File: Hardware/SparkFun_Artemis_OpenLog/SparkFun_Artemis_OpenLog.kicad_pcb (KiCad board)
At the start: 4 copper layers, 30.5 x 30.5 mm, 88 parts, among them J11 Qwiic_RA, J14 SWD, J2 Conn_01x02, J3 Conn_01x02, J4 Conn_01x06, J5 JST_2mm_LiPo, J6 MICRO-SD, J7 Conn_01x01, J8 USB_C_Receptacle, Q2 DMG2305UX, SW3 SMD_4.6x2.8mm_h2.5mm, U1 3.0V Supervisor, U10 CH340E, U2 MCP73831, U3 AP2112K-3.3, U4 AP2112K-3.3, U5 BNO086, U8 Artemis Module, Y1 32.768kHz, Y3 32.768kHz

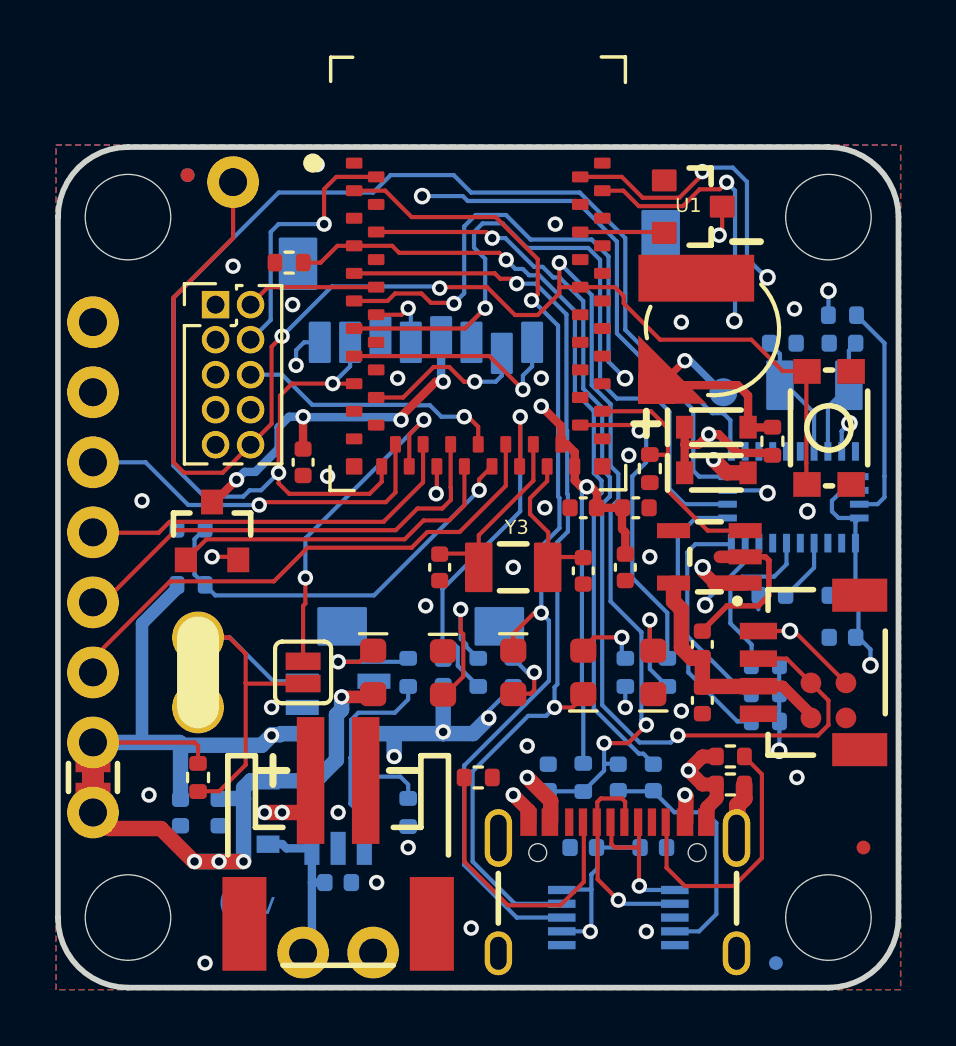
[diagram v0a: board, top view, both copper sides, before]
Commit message: Updates microSD - save point
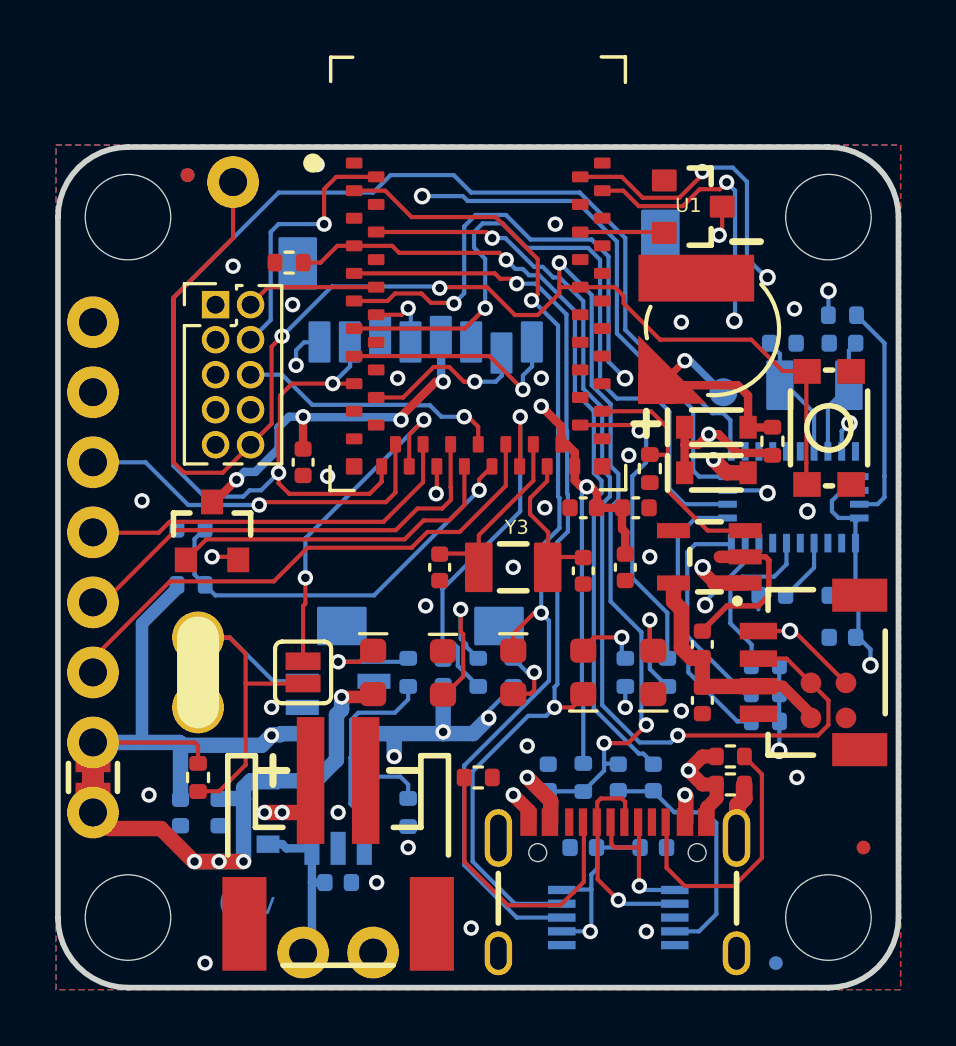
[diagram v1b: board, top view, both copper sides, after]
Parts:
- J6: value MICRO-SD -> microSD; footprint MICRO-SD-SOCKET -> SparkFun-Connector:microSD_SOCKET
- moved J6 9.97 mm to (148.5, 100.4)
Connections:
- C46 pad 1: Net-(Q2-D) -> Net-(J6-VDD)
- Q2 pad 3: Net-(Q2-D) -> Net-(J6-VDD)
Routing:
- net Net-(Q2-D): track 13.6 -> 0.00 mm, vias 4 -> 0
- net Net-(J6-VDD): track 0.00 -> 13.6 mm, vias 0 -> 4
